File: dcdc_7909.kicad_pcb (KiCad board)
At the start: 2 copper layers, 36.8 x 26 mm, 28 parts, among them J1 V_IN, J2 G_IN, J3 +10V, J4 G_OUT, J5 -10V, U1 TMR6, U2 LT3045xMSE, U3 LT3094xMSE

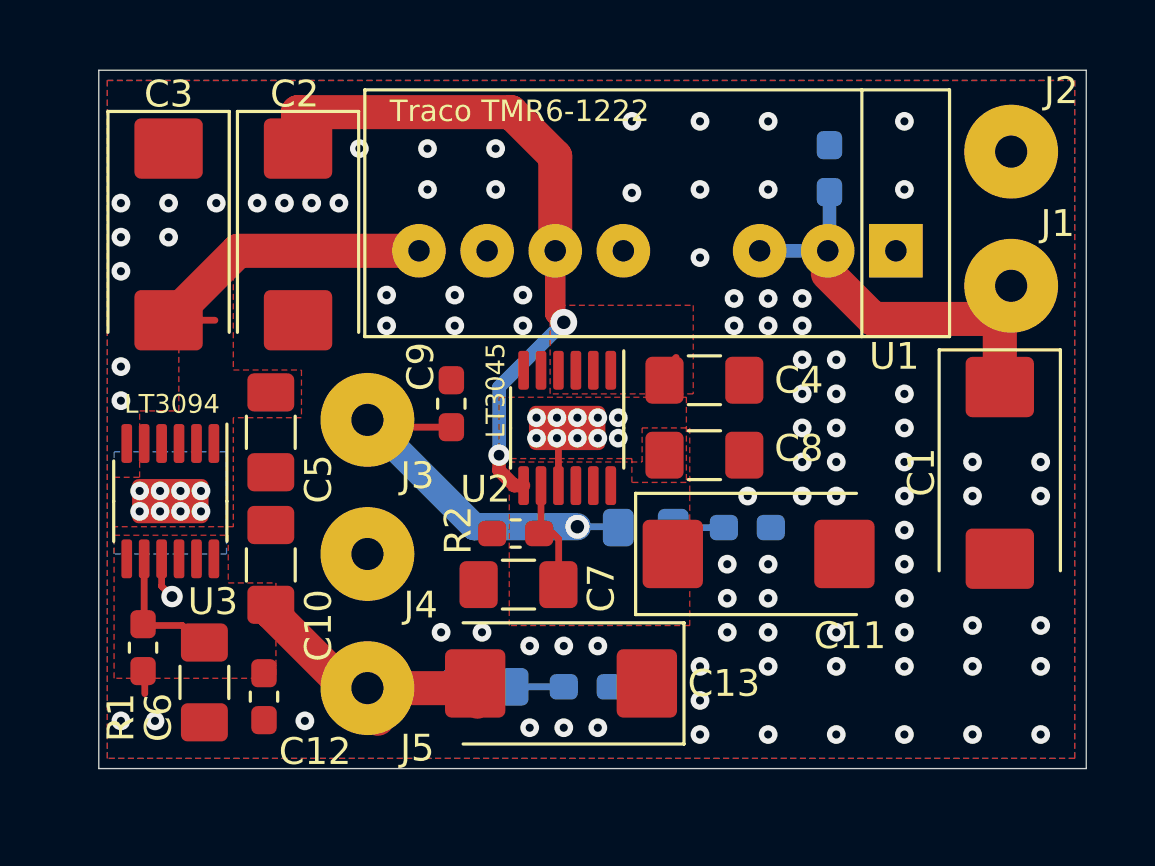
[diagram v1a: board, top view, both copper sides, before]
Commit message: V2 PCB almost finished.
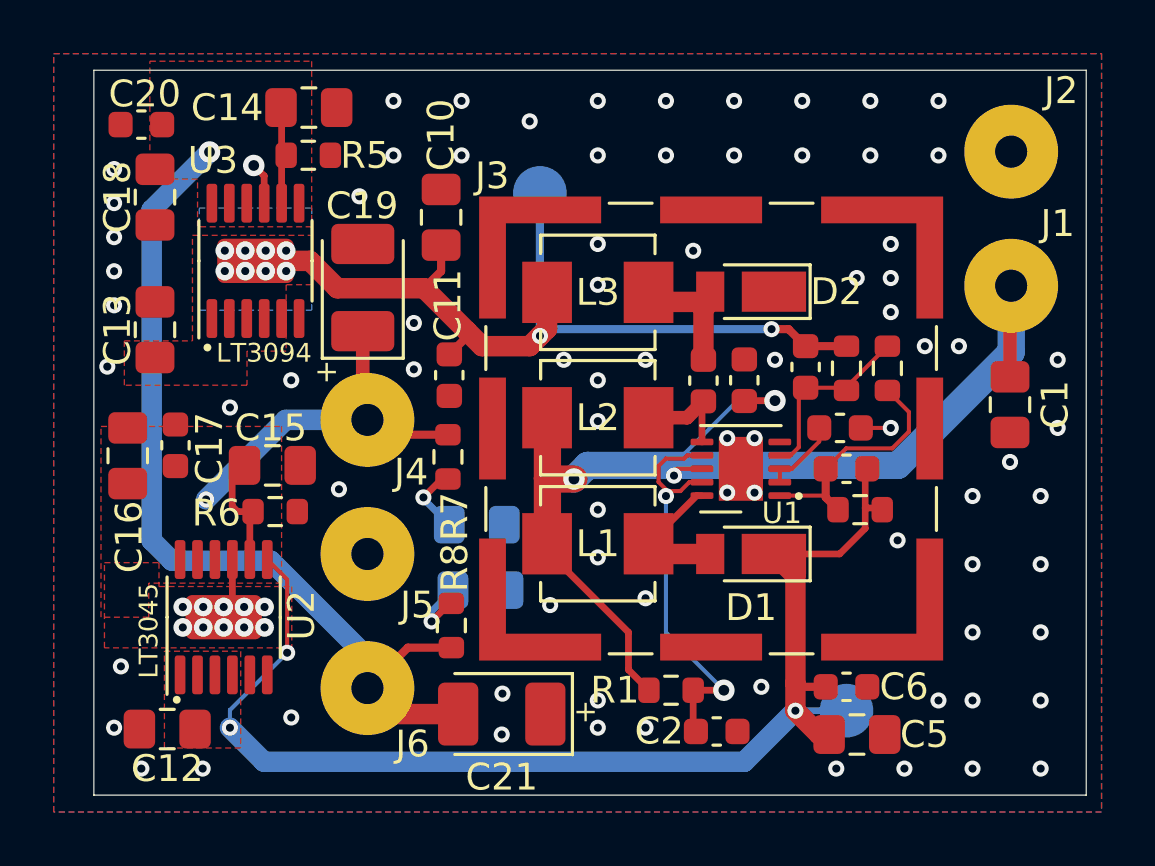
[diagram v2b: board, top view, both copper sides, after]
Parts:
- removed the C13 at (96.4, 76.8)
- removed the C14 at (106.4, 57.6)
- added C10: 22u, Capacitor_SMD:C_0805_2012Metric_Pad1.18x1.45mm_HandSolder, F.Cu at (91.9, 59.5)
- added C19: C_Polarized_Small, Capacitor_Tantalum_SMD:CP_EIA-3528-21_Kemet-B_Pad1.50x2.35mm_HandSolder, F.Cu at (89.0, 62.1)
- added C21: C_Polarized_Small, Capacitor_Tantalum_SMD:CP_EIA-3528-21_Kemet-B_Pad1.50x2.35mm_HandSolder, F.Cu at (94.2, 78.0)
- added C4: 2200p, Capacitor_SMD:C_0603_1608Metric, F.Cu at (107.1, 68.8)
- added C5: 22u, Capacitor_SMD:C_0805_2012Metric_Pad1.18x1.45mm_HandSolder, F.Cu at (107.5, 78.7)
- added C6: 10n, Capacitor_SMD:C_0603_1608Metric, F.Cu at (107.1, 77.0)
- added C7: 10u X7R, Capacitor_SMD:C_0603_1608Metric, F.Cu at (101.7, 65.5)
- added C8: 10u X7R, Capacitor_SMD:C_0603_1608Metric, F.Cu at (103.3, 65.5)
- added C9: 470p, Capacitor_SMD:C_0603_1608Metric, F.Cu at (105.5, 65.0)
- added D1: D_Schottky, Diode_SMD:D_PowerDI-123, F.Cu at (103.5, 72.0)
- added D2: D_Schottky, Diode_SMD:D_PowerDI-123, F.Cu at (103.5, 62.2)
- added J3: RFShield_OnePiece, RF_Shielding:Laird_Technologies_BMI-S-102_16.50x16.50mm, F.Cu at (102.0, 67.3)
- added L1: 10u, Inductor_SMD:L_Vishay_IHLP-1616, F.Cu at (97.8, 71.6)
- added L2: 10u, Inductor_SMD:L_Vishay_IHLP-1616, F.Cu at (97.8, 66.9)
- added L3: 10u, Inductor_SMD:L_Vishay_IHLP-1616, F.Cu at (97.8, 62.3)
- added R1: 20k, Resistor_SMD:R_0603_1608Metric, F.Cu at (100.5, 77.1)
- added R2: 10k, Resistor_SMD:R_0603_1608Metric, F.Cu at (107.6, 70.4)
- added R3: 1.58k, Resistor_SMD:R_0603_1608Metric, F.Cu at (108.6, 65.1)
- added R4: 10k, Resistor_SMD:R_0603_1608Metric, F.Cu at (107.1, 65.1)
- added TP1: +10.5V, TestPoint:TestPoint_Pad_D2.0mm, B.Cu at (107.1, 77.9)
- added TP2: -10.5V, TestPoint:TestPoint_Pad_D2.0mm, B.Cu at (95.6, 58.5)
- C1: value 100u 25v -> 22u; footprint Capacitor_Tantalum_SMD:CP_EIA-7343-31_Kemet-D_Pad2.25x2.55mm_HandSolder -> Capacitor_SMD:C_0805_2012Metric_Pad1.18x1.45mm_HandSolder
- C11: value 100u 16V -> 10n; footprint Capacitor_Tantalum_SMD:CP_EIA-7343-31_Kemet-D_Pad2.25x2.55mm_HandSolder -> Capacitor_SMD:C_0603_1608Metric
- C12: renamed from C4; footprint Capacitor_SMD:C_1206_3216Metric_Pad1.42x1.75mm_HandSolder -> Capacitor_SMD:C_0805_2012Metric_Pad1.18x1.45mm_HandSolder
- C13: renamed from C5; footprint Capacitor_SMD:C_1206_3216Metric_Pad1.42x1.75mm_HandSolder -> Capacitor_SMD:C_0805_2012Metric_Pad1.18x1.45mm_HandSolder
- C14: renamed from C6; footprint Capacitor_SMD:C_1206_3216Metric_Pad1.42x1.75mm_HandSolder -> Capacitor_SMD:C_0805_2012Metric_Pad1.18x1.45mm_HandSolder
- C15: renamed from C7; footprint Capacitor_SMD:C_1206_3216Metric_Pad1.42x1.75mm_HandSolder -> Capacitor_SMD:C_0805_2012Metric_Pad1.18x1.45mm_HandSolder
- C16: renamed from C8; footprint Capacitor_SMD:C_1206_3216Metric_Pad1.42x1.75mm_HandSolder -> Capacitor_SMD:C_0805_2012Metric_Pad1.18x1.45mm_HandSolder
- C17: renamed from C9; footprint Capacitor_SMD:C_0603_1608Metric_Pad1.05x0.95mm_HandSolder -> Capacitor_SMD:C_0603_1608Metric
- C18: renamed from C10; footprint Capacitor_SMD:C_1206_3216Metric_Pad1.42x1.75mm_HandSolder -> Capacitor_SMD:C_0805_2012Metric_Pad1.18x1.45mm_HandSolder
- C2: value 100u 16V -> 10u X7R; footprint Capacitor_Tantalum_SMD:CP_EIA-7343-31_Kemet-D_Pad2.25x2.55mm_HandSolder -> Capacitor_SMD:C_0603_1608Metric
- C20: renamed from C12; footprint Capacitor_SMD:C_0603_1608Metric_Pad1.05x0.95mm_HandSolder -> Capacitor_SMD:C_0603_1608Metric
- C3: value 100u 16V -> 100n X7R; footprint Capacitor_Tantalum_SMD:CP_EIA-7343-31_Kemet-D_Pad2.25x2.55mm_HandSolder -> Capacitor_SMD:C_0603_1608Metric
- D3: renamed from D1; footprint LED_SMD:LED_0603_1608Metric_Pad1.05x0.95mm_HandSolder -> LED_SMD:LED_0805_2012Metric_Pad1.15x1.40mm_HandSolder
- D4: renamed from D2; footprint LED_SMD:LED_0603_1608Metric_Pad1.05x0.95mm_HandSolder -> LED_SMD:LED_0805_2012Metric_Pad1.15x1.40mm_HandSolder
- R5: renamed from R1; value 100k -> 100k 1%; footprint Resistor_SMD:R_0603_1608Metric_Pad1.05x0.95mm_HandSolder -> Resistor_SMD:R_0603_1608Metric
- R6: renamed from R2; value 100k -> 100k 1%; footprint Resistor_SMD:R_0603_1608Metric_Pad1.05x0.95mm_HandSolder -> Resistor_SMD:R_0603_1608Metric
- R7: renamed from R3; value 820 -> 1k; footprint Resistor_SMD:R_0805_2012Metric_Pad1.15x1.40mm_HandSolder -> Resistor_SMD:R_0603_1608Metric; moved to F.Cu
- R8: renamed from R4; value 820 -> 1k; footprint Resistor_SMD:R_0805_2012Metric_Pad1.15x1.40mm_HandSolder -> Resistor_SMD:R_0603_1608Metric; moved to F.Cu
- U1: value TMR6 -> LT3471; footprint marcin_library:Traco_TMR6 -> Package_DFN_QFN:DFN-10-1EP_3x3mm_P0.5mm_EP1.65x2.38mm
- moved C3 26.1 mm to (106.8, 67.3), turned to 0 degrees
- moved C2 24.2 mm to (102.2, 78.6), turned to 0 degrees
- moved C12 23.9 mm to (81.7, 78.5), turned to 180 degrees
- moved C20 21.8 mm to (80.8, 56.0), turned to 180 degrees
- moved C14 21.8 mm to (87.0, 55.4), turned to 0 degrees
- moved C16 21.5 mm to (80.3, 68.3), turned to 90 degrees
- moved R5 19.4 mm to (87.0, 57.1), turned to 0 degrees
- moved U2 14.6 mm to (83.8, 74.4), turned to 90 degrees
- moved C18 14.4 mm to (81.3, 58.7), turned to -90 degrees
- moved C11 13.3 mm to (92.3, 65.3), turned to -90 degrees
- moved C17 10.4 mm to (82.0, 68.0)
- moved C15 10.2 mm to (85.7, 68.7), turned to 0 degrees
- moved D3 10.1 mm to (93.3, 70.9)
- moved U1 9.97 mm to (103.1, 68.8)
- moved U3 9.50 mm to (85.0, 61.1), turned to 90 degrees
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- renumbered J3 to J4, J4 to J5, J5 to J6
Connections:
- net -12V renamed /-10V
- C11 pad 1: +12V -> /-10.5V
- C12 pad 1: Net-(C2-Pad1) -> /+10.5V
- C13 pad 1: Net-(C3-Pad2) -> /-10.5V
- C16 pad 1: +12V -> /+10V
- C17 pad 1: +12V -> /+10V
- C3 pad 1: GND -> Net-(C3-Pad1)
- C3 pad 2: Net-(C3-Pad2) -> GND
- J4 pad 1: +12V -> /+10V
- R7 pad 1: +12V -> /+10V
- U1 pad 1: GND -> Net-(C4-Pad2)
- U1 pad 2: VCC -> Net-(C3-Pad1)
- U1 pad 3: VCC -> Net-(C3-Pad1)
- U1 pad 5: Net-(U1-Pad5) -> GND
- U1 pad 6: Net-(C2-Pad1) -> Net-(C7-Pad1)
- U1 pad 7: GND -> Net-(C2-Pad1)
- U1 pad 8: Net-(C3-Pad2) -> VCC
- U2 pad 1: Net-(C2-Pad1) -> /+10.5V
- U2 pad 10: +12V -> /+10V
- U2 pad 11: +12V -> /+10V
- U2 pad 12: +12V -> /+10V
- U2 pad 2: Net-(C2-Pad1) -> /+10.5V
- U2 pad 3: Net-(C2-Pad1) -> /+10.5V
- U2 pad 4: Net-(C2-Pad1) -> /+10.5V
- U2 pad 5: Net-(U2-Pad5) -> unconnected-(U2-Pad5)
- U2 pad 7: Net-(C2-Pad1) -> /+10.5V
- U3 pad 1: Net-(C3-Pad2) -> /-10.5V
- U3 pad 13: Net-(C3-Pad2) -> /-10.5V
- U3 pad 2: Net-(C3-Pad2) -> /-10.5V
- U3 pad 3: Net-(C3-Pad2) -> /-10.5V
- U3 pad 4: Net-(U3-Pad4) -> unconnected-(U3-Pad4)
- U3 pad 5: Net-(C3-Pad2) -> /-10.5V
- U3 pad 7: Net-(U3-Pad7) -> unconnected-(U3-Pad7)
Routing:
- net /+10.5V: track 0.00 -> 47.4 mm, vias 0 -> 3
- net /-10.5V: track 0.00 -> 34.0 mm, vias 0 -> 10
- net VCC: track 16.9 -> 44.4 mm, vias 0 -> 3
- net /-10V: track 13.6 -> 33.9 mm, vias 0 -> 1
- net +12V: track 14.3 -> 0.00 mm, vias 1 -> 0
- net /+10V: track 0.00 -> 12.8 mm, vias 0 -> 1
- net Net-(C3-Pad2): track 12.1 -> 0.00 mm, vias 8 -> 0
- net Net-(C2-Pad1): track 26.3 -> 15.3 mm
- net Net-(C4-Pad2): track 0.00 -> 9.00 mm
- net Net-(C9-Pad2): track 0.00 -> 7.00 mm
- net Net-(D1-Pad2): track 0.00 -> 5.19 mm
- net Net-(C7-Pad2): track 0.00 -> 4.71 mm
- net Net-(C7-Pad1): track 0.00 -> 3.82 mm
- net Net-(C3-Pad1): track 0.00 -> 2.90 mm
- net Net-(C14-Pad1): track 5.02 -> 3.57 mm
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- added copper zone on F.Cu, net /+10.5V
- added copper zone on F.Cu, net /+10V
- added copper zone on B.Cu, net /-10.5V
- added copper zone on F.Cu, net /-10.5V
- removed copper zone on F.Cu, net +12V
- removed copper zone on F.Cu, net Net-(C2-Pad1)
- removed copper zone on B.Cu, net Net-(C3-Pad2)
- removed copper zone on F.Cu, net Net-(C3-Pad2)
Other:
- board size 36.8 x 26 mm -> 37 x 27 mm
- net class Default removed
- board text added: "+"
- board text added: "+10V"
- board text added: "-10V"
- board text added: "Alpine 7909 DC/DC v2.0 (c) M. Dymczyk 07.2023"
- board text removed: "Alpine 7909 DC/DC v1.1 (c) M. Dymczyk 04.2020"
- board text removed: "Traco TMR6-1222"
